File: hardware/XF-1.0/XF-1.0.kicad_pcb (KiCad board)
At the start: 2 copper layers, 100.3 x 111.8 mm, 23 parts, among them CN1 Conn_01x02, CN2 Conn_01x02, CN3 Conn_01x03, CN4 Conn_01x03, CN5 Conn_01x02, CN6 Conn_01x03, CN7 Conn_01x02

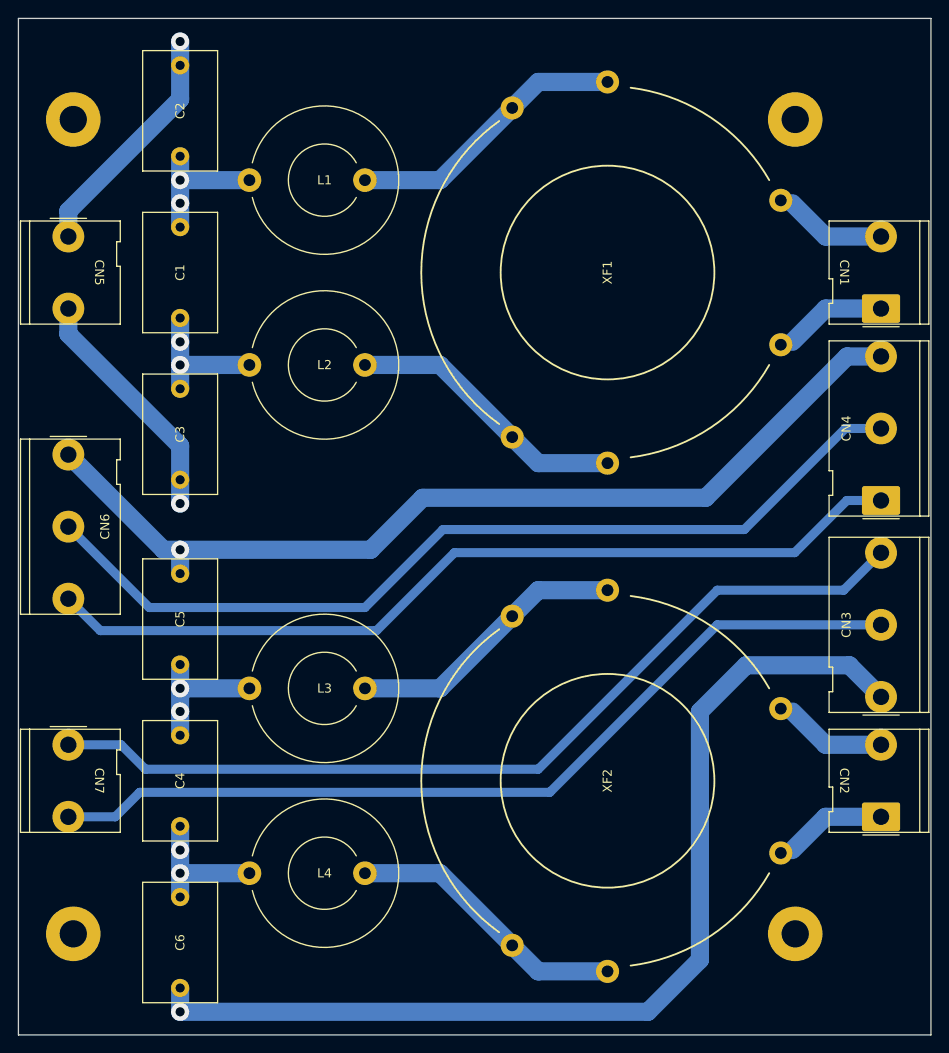
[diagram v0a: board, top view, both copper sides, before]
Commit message: modified:   .DS_Store 	new file:   hardware/.~Request PO 20250807.xlsx 	new file:   hardware/CTL-3.0/.~BoM.xlsx 	modified:   hardware/CTL-3.0/BoM.xlsx 	deleted:    hardware/PS-2.0/PS-2.0-backups/PS-2.0-2025-07-26_112315.zip 	deleted:    hardware/PS-2.0/PS-2.0-backups/PS-2.0-2025-07-26_113619.zip 	deleted:    hardware/PS-2.0/PS-2.0-backups/PS-2.0-2025-07-26_114654.zip 	deleted:    hardware/PS-2.0/PS-2.0-backups/PS-2.0-2025-08-06_121001.zip 	new file:   hardware/PS-2.0/PS-2.0-backups/PS-2.0-2025-08-07_142024.zip 	new file:   hardware/PS-2.0/PS-2.0-backups/PS-2.0-2025-08-07_143133.zip 	new file:   hardware/PS-2.0/PS-2.0-backups/PS-2.0-2025-08-07_145326.zip 	new file:   hardware/PS-2.0/PS-2.0-backups/PS-2.0-2025-08-07_160132.zip 	new file:   hardware/PS-2.0/PS-2.0-backups/PS-2.0-2025-08-07_161316.zip 	new file:   hardware/PS-2.0/_autosave-PS-2.0.kicad_pcb 	new file:   hardware/PS-2.0/~_autosave-PS-2.0.kicad_pcb.lck 	new file:   hardware/Request PO 20250807 1029.xlsx 	deleted:    hardware/XF-1.0/XF-1.0-backups/XF-1.0-2025-07-15_152320.zip 	deleted:    hardware/XF-1.0/XF-1.0-backups/XF-1.0-2025-07-15_154638.zip 	deleted:    hardware/XF-1.0/XF-1.0-backups/XF-1.0-2025-07-16_140719.zip 	deleted:    hardware/XF-1.0/XF-1.0-backups/XF-1.0-2025-07-17_145542.zip 	deleted:    hardware/XF-1.0/XF-1.0-backups/XF-1.0-2025-07-17_150101.zip 	deleted:    hardware/XF-1.0/XF-1.0-backups/XF-1.0-2025-07-17_150621.zip 	deleted:    hardware/XF-1.0/XF-1.0-backups/XF-1.0-2025-07-17_151256.zip 	new file:   hardware/XF-1.0/XF-1.0-backups/XF-1.0-2025-08-07_145812.zip 	new file:   hardware/XF-1.0/XF-1.0-backups/XF-1.0-2025-08-07_150444.zip 	new file:   hardware/XF-1.0/XF-1.0-backups/XF-1.0-2025-08-07_151358.zip 	new file:   hardware/XF-1.0/XF-1.0-backups/XF-1.0-2025-08-07_152043.zip 	new file:   hardware/XF-1.0/XF-1.0-backups/XF-1.0-2025-08-07_153427.zip 	new file:   hardware/XF-1.0/XF-1.0-backups/XF-1.0-2025-08-07_155906.zip 	modified:   hardware/XF-1.0/XF-1.0.kicad_pcb 	modified:   hardware/XF-1.0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
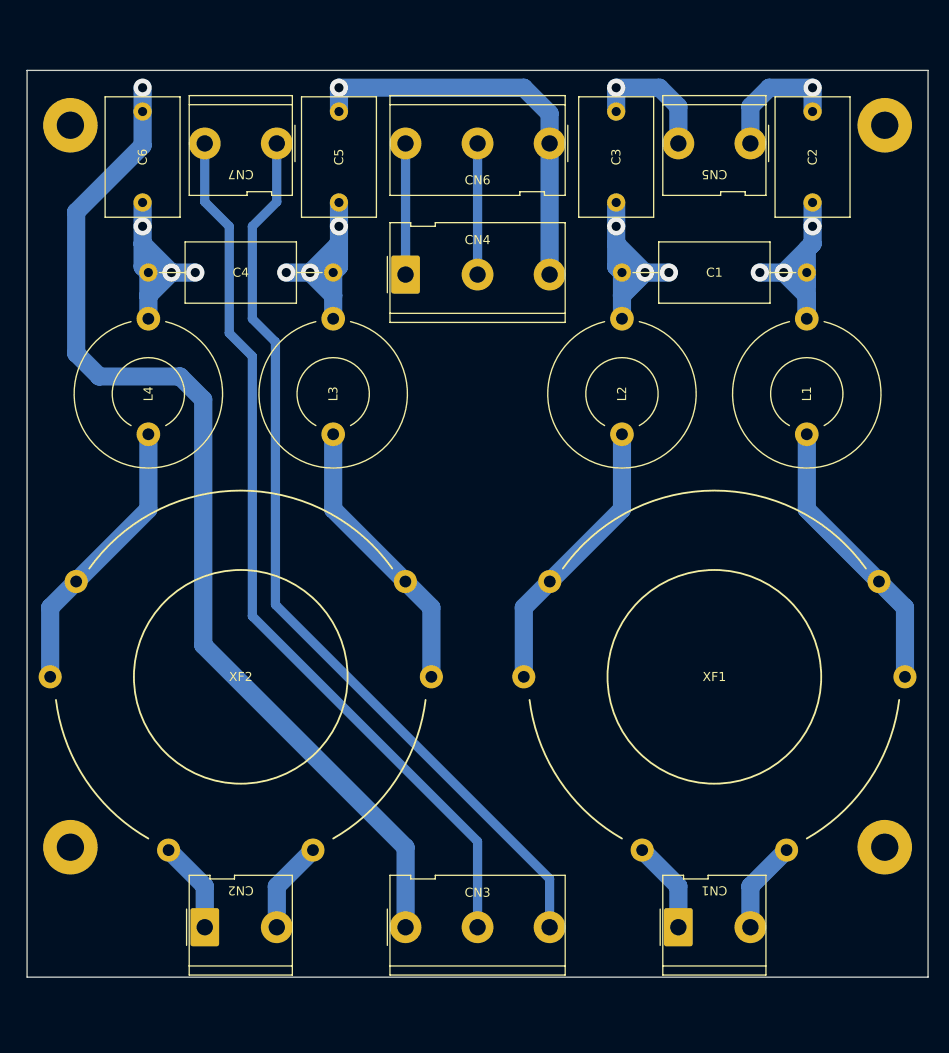
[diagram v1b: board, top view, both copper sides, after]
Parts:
- C1, C4: footprint Capacitor_THT:C_Rect_L13.0mm_W8.0mm_P10.00mm_FKS3_FKP3_MKS4 -> Capacitor_THT:C_Axial_L12.0mm_D6.5mm_P20.00mm_Horizontal
- moved H1 89.2 mm to (120.7, 52.4), turned to -90 degrees
- moved H2 88.9 mm to (31.1, 52.4), turned to -90 degrees
- moved H4 80.6 mm to (120.7, 131.8), turned to -90 degrees
- moved H3 80.3 mm to (31.1, 131.8), turned to -90 degrees
- moved C6 76.5 mm to (39.1, 60.9), turned to 90 degrees
- moved CN5 75.7 mm to (105.9, 54.4), turned to 180 degrees
- moved CN2 75.3 mm to (45.9, 140.6), turned to 0 degrees
- moved CN1 71.6 mm to (98.0, 140.6), turned to 0 degrees
- moved CN7 70.0 mm to (53.8, 54.4), turned to 180 degrees
- moved C2 69.7 mm to (112.7, 60.9)
- moved C1 68.9 mm to (111.9, 68.6), turned to 180 degrees
- moved CN6 63.0 mm to (83.8, 54.4), turned to 180 degrees
- moved CN3 58.1 mm to (68.0, 140.6), turned to 0 degrees
- moved L1 58.0 mm to (112.1, 81.9), turned to 90 degrees
- moved CN4 57.9 mm to (68.0, 68.8), turned to 0 degrees
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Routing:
- net Net-(CN4-Pin_2): track 101.2 -> 14.4 mm
- net Net-(CN4-Pin_1): track 96.7 -> 14.4 mm
- net Net-(CN4-Pin_3): track 105.1 -> 44.7 mm
- net Net-(C1-Pad1): track 15.4 -> 30.1 mm, vias 2 -> 3
- net Net-(CN5-Pin_2): track 26.5 -> 14.4 mm
- net Net-(CN5-Pin_1): track 26.5 -> 14.4 mm
- net Net-(C4-Pad1): track 15.4 -> 26.3 mm, vias 2 -> 3
- net Net-(C1-Pad2): track 15.4 -> 26.3 mm, vias 2 -> 3
- net Net-(C4-Pad2): track 15.4 -> 26.3 mm, vias 2 -> 3
- net Net-(CN3-Pin_1): track 112.9 -> 115.5 mm
- net Net-(CN2-Pin_1): track 11.3 -> 10.1 mm
- net Net-(CN1-Pin_1): track 11.3 -> 10.1 mm
- net Net-(CN2-Pin_2): track 11.3 -> 10.1 mm
- net Net-(CN1-Pin_2): track 11.3 -> 10.1 mm
- net Net-(CN3-Pin_3): track 100.3 -> 100.8 mm
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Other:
- board size 100.3 x 111.8 mm -> 99.1 x 99.7 mm
